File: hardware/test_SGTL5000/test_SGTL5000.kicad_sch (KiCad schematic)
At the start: 18 parts

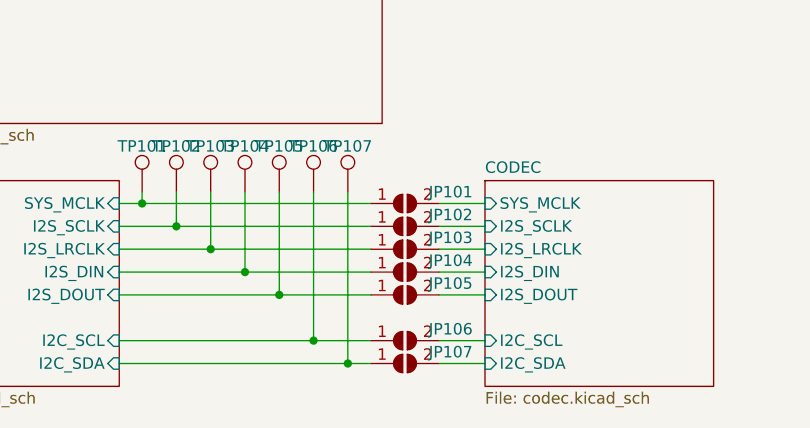
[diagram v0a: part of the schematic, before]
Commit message: routing
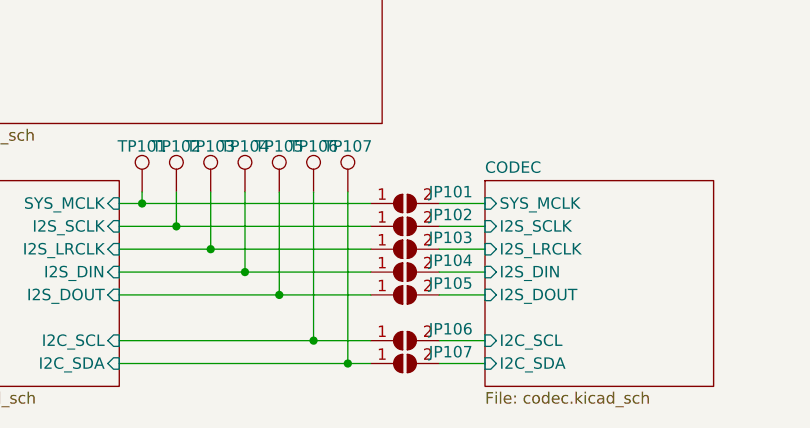
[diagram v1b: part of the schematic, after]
